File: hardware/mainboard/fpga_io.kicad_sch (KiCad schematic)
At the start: 25 parts

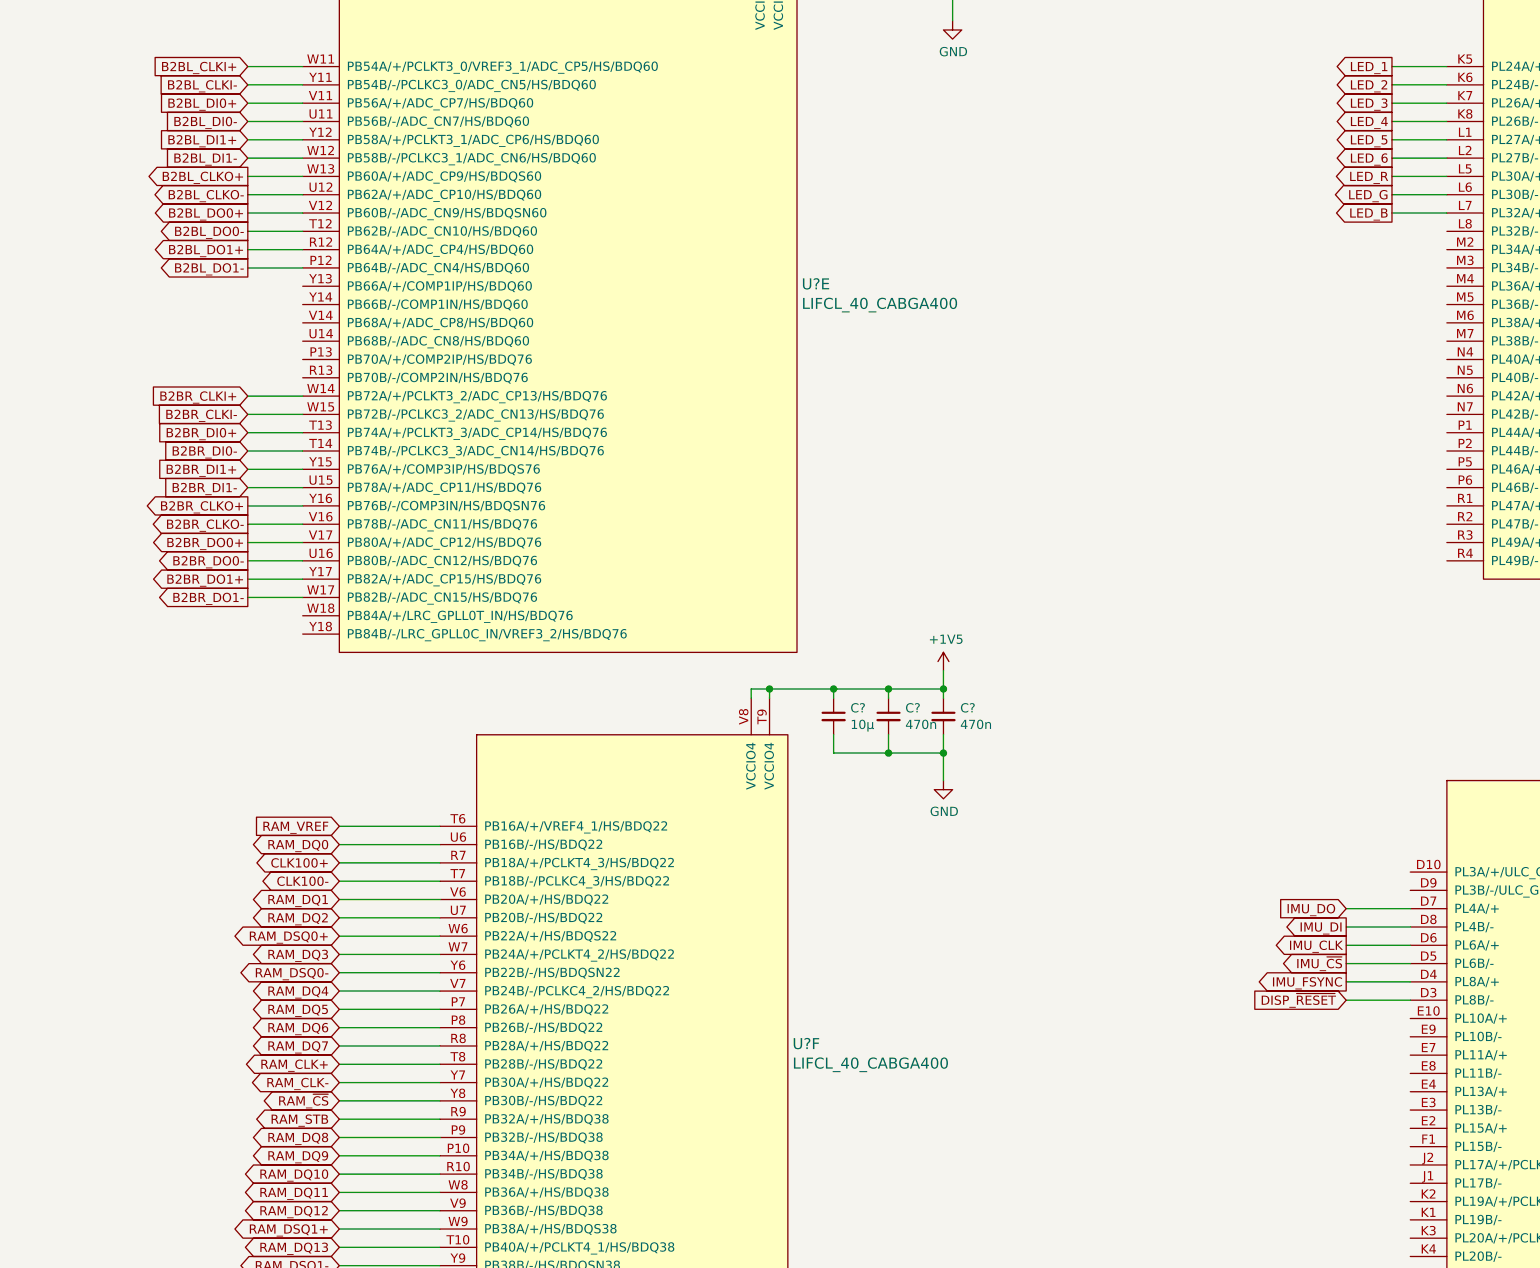
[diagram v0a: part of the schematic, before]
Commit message: Misc bits
Signed-off-by: David Shah <dave@ds0.me>
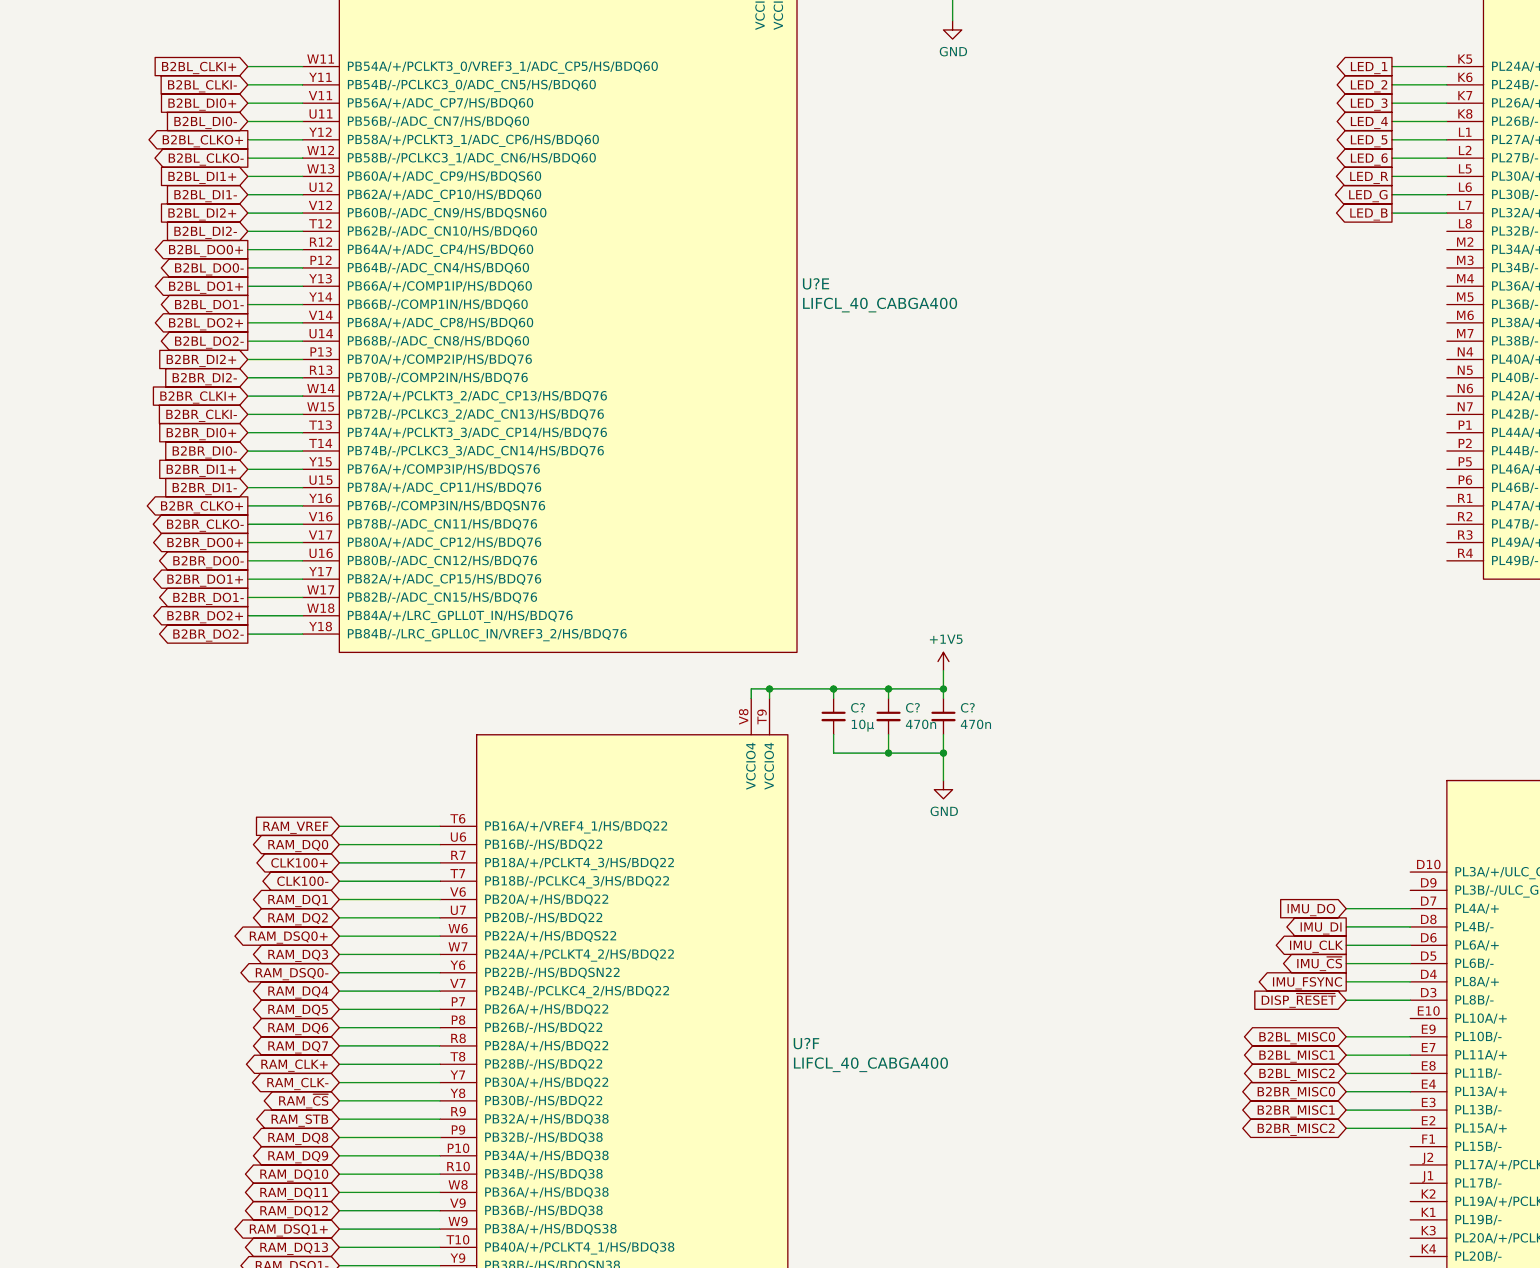
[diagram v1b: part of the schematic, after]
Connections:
- net B2BL_CLKO+: now also U?.Y12 (PB58A/+/PCLKT3_1/ADC_CP6/HS/BDQ60); no longer U?.W13 (PB60A/+/ADC_CP9/HS/BDQS60)
- net B2BL_CLKO-: now also U?.W12 (PB58B/-/PCLKC3_1/ADC_CN6/HS/BDQ60); no longer U?.U12 (PB62A/+/ADC_CP10/HS/BDQ60)
- net B2BL_DI1+: now also U?.W13 (PB60A/+/ADC_CP9/HS/BDQS60); no longer U?.Y12 (PB58A/+/PCLKT3_1/ADC_CP6/HS/BDQ60)
- net B2BL_DI1-: now also U?.U12 (PB62A/+/ADC_CP10/HS/BDQ60); no longer U?.W12 (PB58B/-/PCLKC3_1/ADC_CN6/HS/BDQ60)
- net B2BL_DO0+: now also U?.R12 (PB64A/+/ADC_CP4/HS/BDQ60); no longer U?.V12 (PB60B/-/ADC_CN9/HS/BDQSN60)
- net B2BL_DO0-: now also U?.P12 (PB64B/-/ADC_CN4/HS/BDQ60); no longer U?.T12 (PB62B/-/ADC_CN10/HS/BDQ60)
- net B2BL_DO1+: now also U?.Y13 (PB66A/+/COMP1IP/HS/BDQ60); no longer U?.R12 (PB64A/+/ADC_CP4/HS/BDQ60)
- net B2BL_DO1-: now also U?.Y14 (PB66B/-/COMP1IN/HS/BDQ60); no longer U?.P12 (PB64B/-/ADC_CN4/HS/BDQ60)
- net B2BR_MISC2: now reaches U?.E2 (PL15A/+)
- net B2BR_MISC1: now reaches U?.E3 (PL13B/-)
- net B2BR_MISC0: now reaches U?.E4 (PL13A/+)
- net B2BL_MISC1: now reaches U?.E7 (PL11A/+)
- net B2BL_MISC2: now reaches U?.E8 (PL11B/-)
- net B2BL_MISC0: now reaches U?.E9 (PL10B/-)
- net B2BR_DI2+: now reaches U?.P13 (PB70A/+/COMP2IP/HS/BDQ76)
- net B2BR_DI2-: now reaches U?.R13 (PB70B/-/COMP2IN/HS/BDQ76)
- net B2BL_DO2-: now reaches U?.U14 (PB68B/-/ADC_CN8/HS/BDQ60)
- net B2BL_DO2+: now reaches U?.V14 (PB68A/+/ADC_CP8/HS/BDQ60)
- net B2BR_DO2+: now reaches U?.W18 (PB84A/+/LRC_GPLL0T_IN/HS/BDQ76)
- net B2BR_DO2-: now reaches U?.Y18 (PB84B/-/LRC_GPLL0C_IN/VREF3_2/HS/BDQ76)
- new net B2BL_DI2+: U?.V12 (PB60B/-/ADC_CN9/HS/BDQSN60)
- new net B2BL_DI2-: U?.T12 (PB62B/-/ADC_CN10/HS/BDQ60)
